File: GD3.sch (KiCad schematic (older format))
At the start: 19 parts, among them IC13 HCPL-316J, IC14 IXDD614PI, P14 CONN_01X03, P15 CONN_01X03

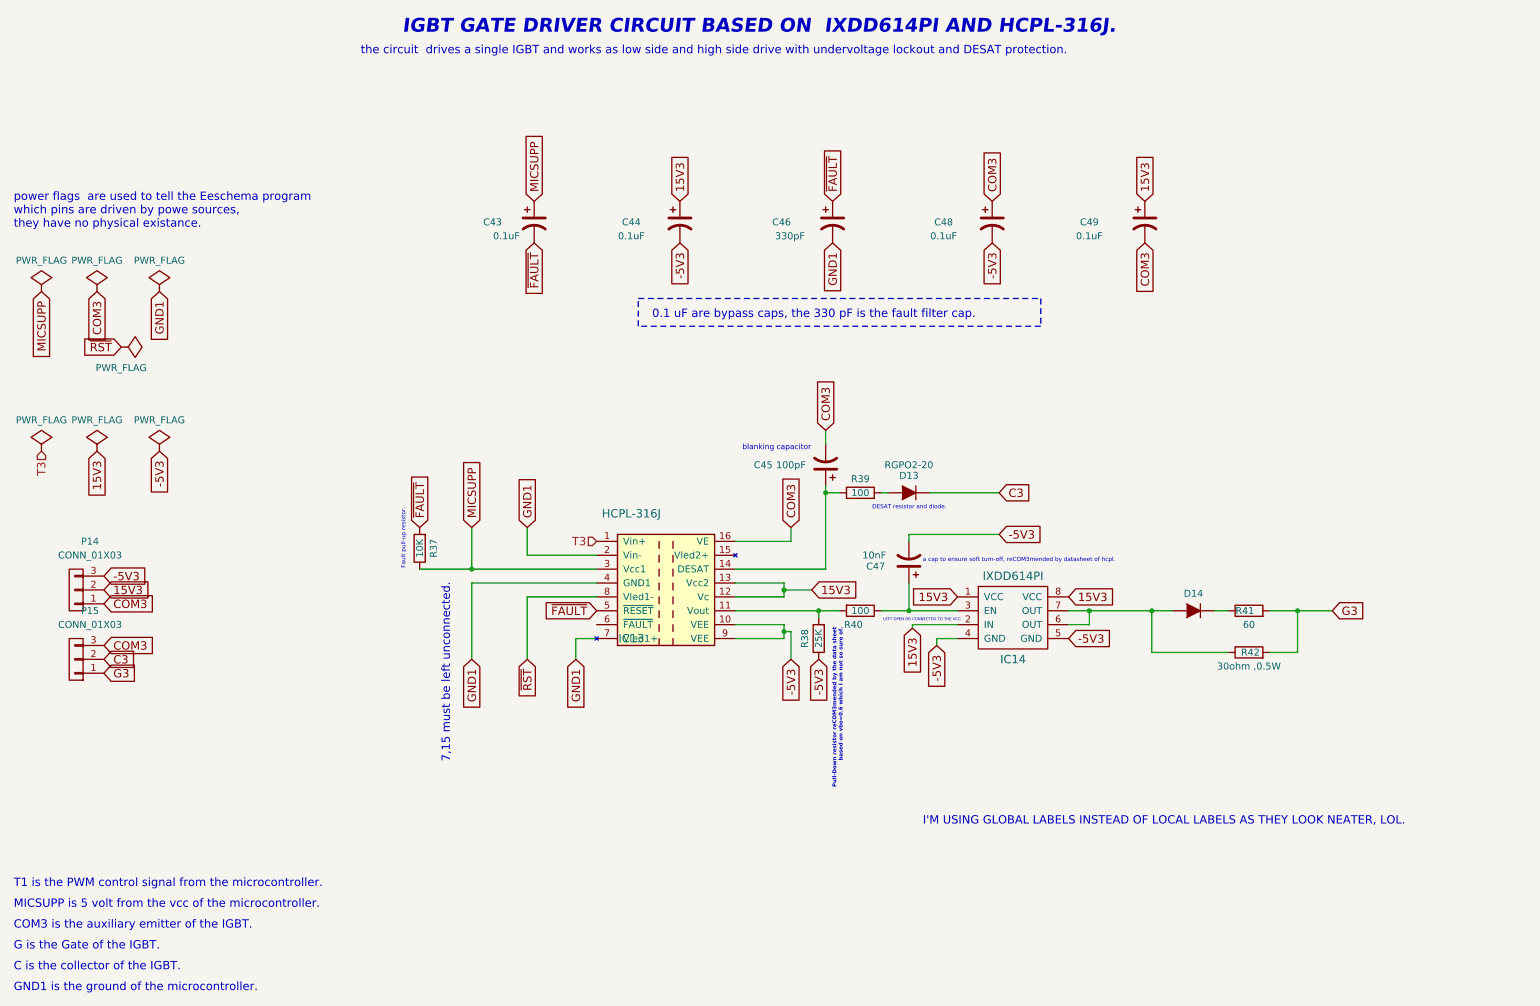
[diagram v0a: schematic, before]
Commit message: packup
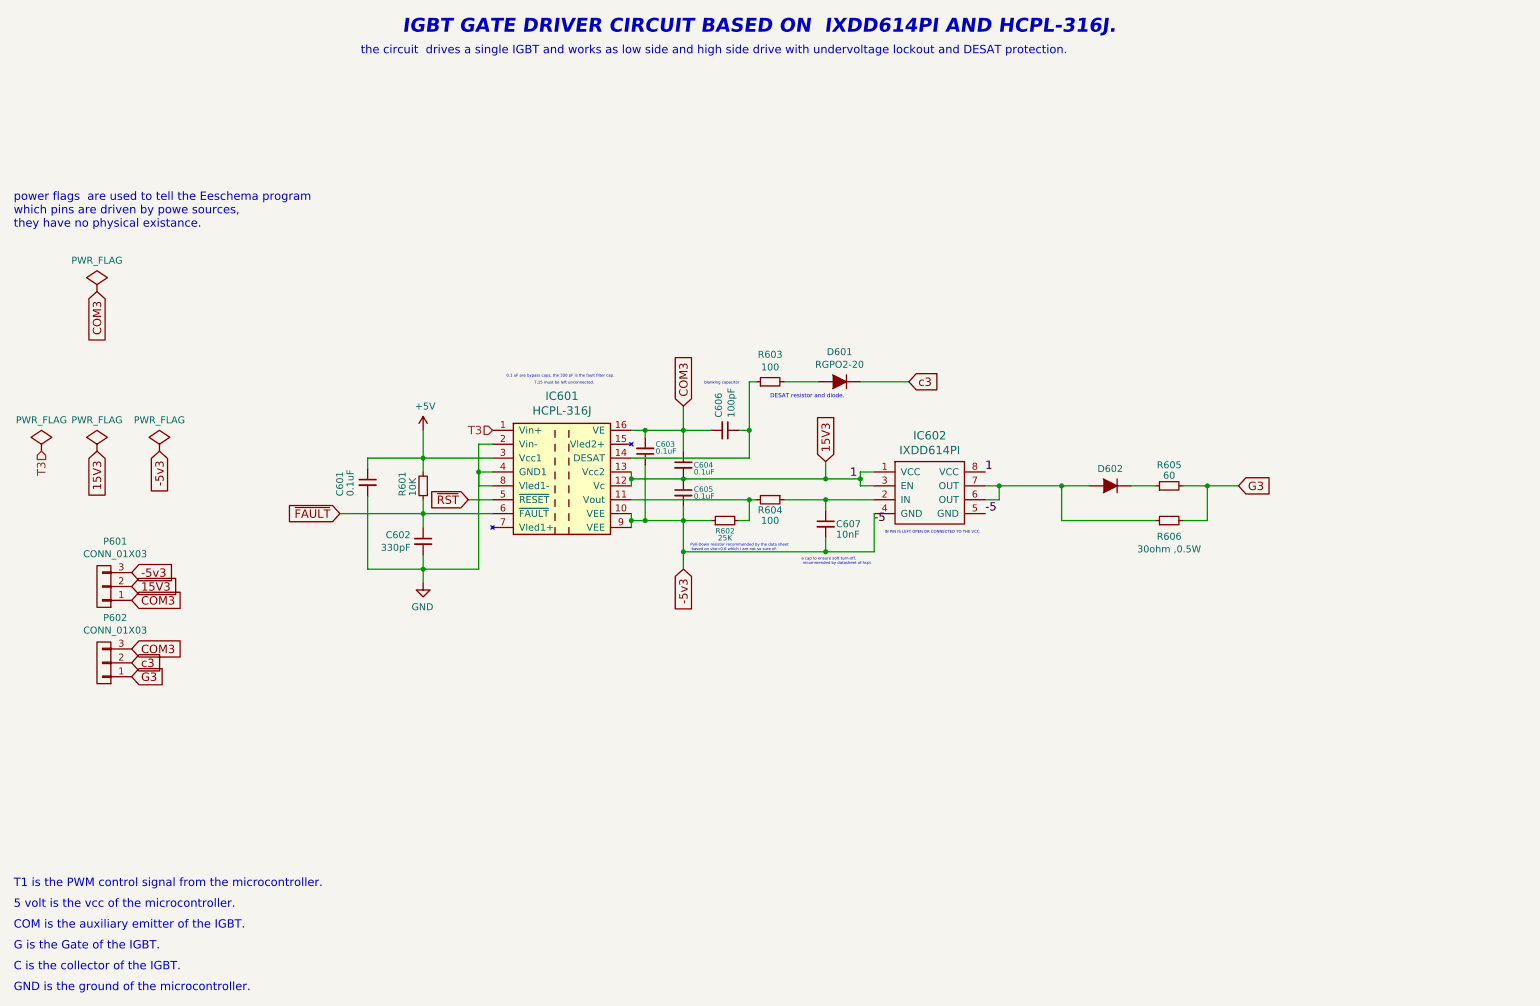
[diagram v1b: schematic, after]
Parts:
- removed C43, C44, C48, C49: 0.1uF, gatedrive:C_Disc, symbol CP1
- removed C45: 100pF, gatedrive:C_Disc, symbol CP1
- removed C46: 330pF, Capacitors_ThroughHole:C_Disc_D3_P2.5, symbol CP1
- removed C47: 10nF, gatedrive:C_Disc, symbol CP1
- removed D13: RGPO2-20, Diodes_ThroughHole:Diode_DO-41_SOD81_Horizontal_RM10, symbol D
- removed D14: ~, Diodes_ThroughHole:Diode_DO-201AD_Horizontal_RM15, symbol D
- removed IC13: HCPL-316J, Housings_SOIC:SOIC-16_7.5x10.3mm_Pitch1.27mm, symbol HCPL-316J
- removed IC14: IXDD614PI, gatedrive:DIP-8_W7.62mm_LongPads, symbol IXDD614PI
- removed P14, P15: CONN_01X03, Pin_Headers:Pin_Header_Angled_1x03, symbol CONN_01X03
- removed R37: 10K, Resistors_ThroughHole:Resistor_Horizontal_RM10mm, symbol R
- removed R38: 25K, Resistors_ThroughHole:Resistor_Horizontal_RM10mm, symbol R
- removed R39, R40: 100, Resistors_ThroughHole:Resistor_Horizontal_RM10mm, symbol R
- removed R41: 60, gatedrive:Resistor_multi, symbol R
- removed R42: 30ohm ,0.5W, gatedrive:Resistor_multi, symbol R
- added C601, C603, C604, C605: 0.1uF, gatedrive:C_Disc, symbol C_Small
- added C602: 330pF, gatedrive:C_Disc, symbol C_Small
- added C606: 100pF, gatedrive:C_Disc, symbol C_Small
- added C607: 10nF, gatedrive:C_Disc, symbol C_Small
- added D601: RGPO2-20, Diodes_ThroughHole:Diode_DO-41_SOD81_Horizontal_RM10, symbol D
- added D602: ~, Diodes_ThroughHole:Diode_DO-201AD_Horizontal_RM15, symbol D
- added IC601: HCPL-316J, Housings_SOIC:SOIC-16_7.5x10.3mm_Pitch1.27mm, symbol HCPL-316J
- added IC602: IXDD614PI, gatedrive:DIP-8_W7.62mm_LongPads, symbol IXDD614PI
- added P601, P602: CONN_01X03, gatedrive:conn, symbol CONN_01X03
- added R601: 10K, Resistors_ThroughHole:Resistor_Horizontal_RM10mm, symbol R_Small
- added R602: 25K, Resistors_ThroughHole:Resistor_Horizontal_RM10mm, symbol R_Small
- added R603, R604: 100, Resistors_ThroughHole:Resistor_Horizontal_RM10mm, symbol R_Small
- added R605: 60, gatedrive:Resistor_multi, symbol R_Small
- added R606: 30ohm ,0.5W, gatedrive:Resistor_multi, symbol R_Small
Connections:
- net 15V3: now also C604.2, C605.1, IC601.12 (Vc), IC601.13 (Vcc2), IC602.1 (VCC), IC602.3 (EN), IC602.8 (VCC), P601.2 (P2)
- net COM3: now also C603.2, C604.1, C606.2, IC601.16 (VE), P601.1 (P1), P602.3 (P3)
- net G3: now also P602.1 (P1), R605.2, R606.2
- net T3: now also IC601.1 (Vin+)
- net ~FAULT: now also C602.1, IC601.6 (~FAULT), R601.1
- net ~RST: now also IC601.5 (~RESET)
- new net: IC601.11 (Vout), R602.2, R604.2
- new net: C606.1, IC601.14 (DESAT), R603.1
- new net: C607.1, IC602.2 (IN), R604.1
- new net: D601.2 (A), R603.2
- new net: D602.1 (K), R605.1
- new net: D602.2 (A), IC602.6 (OUT), IC602.7 (OUT), R606.1
- new net +5V: C601.1, IC601.3 (Vcc1), R601.2
- new net -5v3: C603.1, C605.2, C607.2, IC601.10 (VEE), IC601.9 (VEE), IC602.4 (GND), IC602.5 (GND), P601.3 (P3), R602.1
- new net GND: C601.2, C602.2, IC601.2 (Vin-), IC601.4 (GND1), IC601.8 (Vled1-)
- new net c3: D601.1 (K), P602.2 (P2)
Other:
- note added: "5 volt is the vcc of the microcontroller.\n"
- note added: "COM is the auxiliary emitter of the IGBT."
- note added: "GND is the ground of the microcontroller.\n"
- note added: "IN PIN IS LEFT OPEN OR CONNECTED TO THE VCC."
- note added: "Pull-Down resistor recommended by the data sheet\n based on vbe=0.6 which I am not so sure of."
- note added: "a cap to ensure soft turn-off,\n recommended by datasheet of hcpl."
- note removed: "COM3 is the auxiliary emitter of the IGBT."
- note removed: "Fault pull-up resistor."
- note removed: "GND1 is the ground of the microcontroller.\n"
- note removed: "I'M USING GLOBAL LABELS INSTEAD OF LOCAL LABELS AS THEY LOOK NEATER, LOL."
- note removed: "LEFT OPEN OR CONNECTED TO THE VCC."
- note removed: "MICSUPP is 5 volt from the vcc of the microcontroller.\n"
- note removed: "Pull-Down resistor reCOM3mended by the data sheet\n based on vbe=0.6 which I am not so sure of."
- note removed: "a cap to ensure soft turn-off, reCOM3mended by datasheet of hcpl."

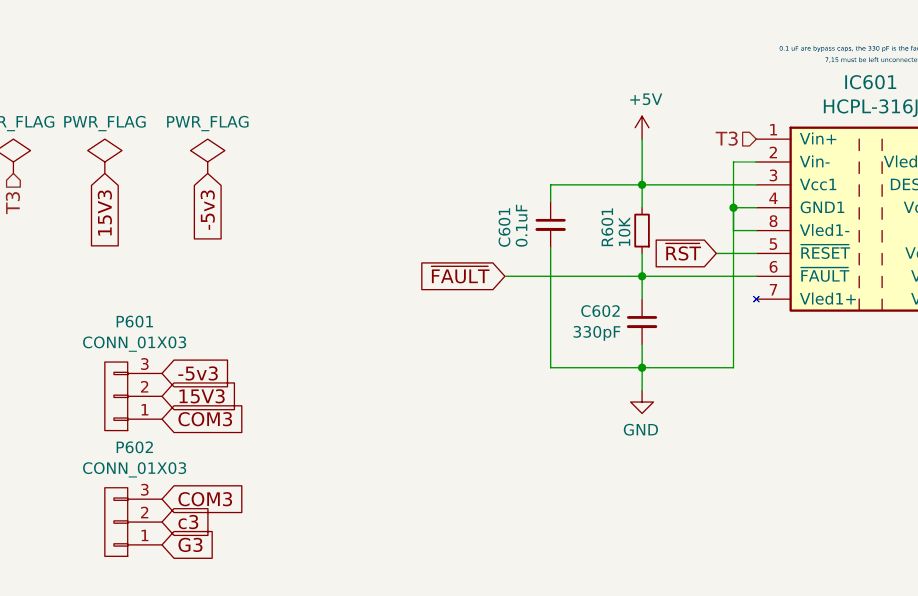
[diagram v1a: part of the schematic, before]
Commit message: parting the protection from the GD
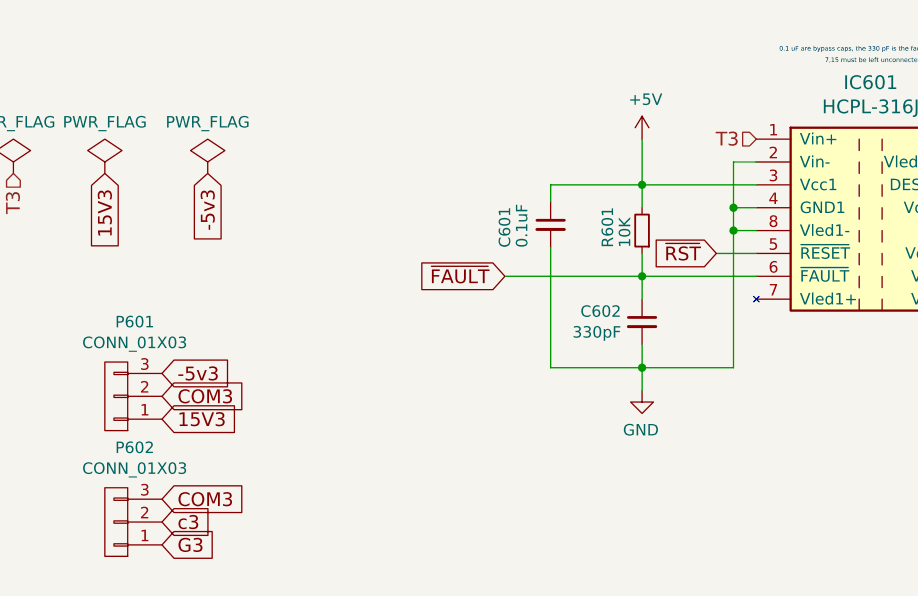
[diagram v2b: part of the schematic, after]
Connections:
- net 15V3: now also P601.1 (P1); no longer P601.2 (P2)
- net COM3: now also P601.2 (P2); no longer P601.1 (P1)
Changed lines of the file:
@@
 IN PIN IS LEFT OPEN OR CONNECTED TO THE VCC.
 $Comp
-L PWR_FLAG #FLG033
+L PWR_FLAG #FLG21
 U 1 1 575FF0FC
 P 1300 3800
-F 0 "#FLG033" H 1300 3895 50  0001 C CNN
+F 0 "#FLG21" H 1300 3895 50  0001 C CNN
 F 1 "PWR_FLAG" H 1300 4024 50  0000 C CNN
 F 2 "" H 1300 3800 50  0000 C CNN
@@
 $EndComp
 $Comp
-L PWR_FLAG #FLG034
+L PWR_FLAG #FLG22
 U 1 1 575FF0FD
 P 1750 3800
-F 0 "#FLG034" H 1750 3895 50  0001 C CNN
+F 0 "#FLG22" H 1750 3895 50  0001 C CNN
 F 1 "PWR_FLAG" H 1750 4024 50  0000 C CNN
 F 2 "" H 1750 3800 50  0000 C CNN
@@
 $EndComp
 $Comp
-L PWR_FLAG #FLG035
+L PWR_FLAG #FLG20
 U 1 1 575FF100
 P 1300 2650
-F 0 "#FLG035" H 1300 2745 50  0001 C CNN
+F 0 "#FLG20" H 1300 2745 50  0001 C CNN
 F 1 "PWR_FLAG" H 1300 2874 50  0000 C CNN
 F 2 "" H 1300 2650 50  0000 C CNN
@@
 $EndComp
 $Comp
-L PWR_FLAG #FLG036
+L PWR_FLAG #FLG19
 U 1 1 575FF101
 P 900 3800
-F 0 "#FLG036" H 900 3895 50  0001 C CNN
+F 0 "#FLG19" H 900 3895 50  0001 C CNN
 F 1 "PWR_FLAG" H 900 4024 50  0000 C CNN
 F 2 "" H 900 3800 50  0000 C CNN
@@
 	5150 4250 5150 4350
 Wire Wire Line
-	5150 3950 5150 4050
-Wire Wire Line
 	6000 3850 5150 3850
 Wire Wire Line
@@
 Wire Wire Line
 	6000 3300 6000 3850
-Connection ~ 7800 4050
 Wire Wire Line
 	7700 4050 8450 4050
@@
 	7700 4150 7800 4150
 Wire Wire Line
-	7800 4150 7800 4050
-Wire Wire Line
 	5150 3650 5725 3650
-Connection ~ 5150 4000
 Wire Wire Line
 	8250 4300 8925 4300
@@
 	-1   0    0    1
 $EndComp
+Text GLabel 1550 4775 2    60   Input ~ 0
+COM3
 Text GLabel 1550 4875 2    60   Input ~ 0
-COM3
-Text GLabel 1550 4775 2    60   Input ~ 0
 15V3
 Text GLabel 1550 5425 2    60   Input ~ 0
@@
 	3975 4150 4150 4150
 $Comp
-L GND #PWR037
+L GND #PWR20
 U 1 1 575FF10A
 P 3650 4750
-F 0 "#PWR037" H 3650 4500 50  0001 C CNN
+F 0 "#PWR20" H 3650 4500 50  0001 C CNN
 F 1 "GND" H 3655 4577 50  0000 C CNN
 F 2 "" H 3650 4750 50  0000 C CNN
@@
 Wire Wire Line
 	4150 3750 4050 3750
-Wire Wire Line
-	4050 3750 4050 4050
-Wire Wire Line
-	4050 4050 4150 4050
-$Comp
-L +5V #PWR038
+$Comp
+L +5V #PWR19
 U 1 1 575FF10B
 P 3650 3650
-F 0 "#PWR038" H 3650 3500 50  0001 C CNN
+F 0 "#PWR19" H 3650 3500 50  0001 C CNN
 F 1 "+5V" H 3665 3823 50  0000 C CNN
 F 2 "" H 3650 3650 50  0000 C CNN
@@
 Connection ~ 3650 4250
 Wire Wire Line
-	4050 3950 4150 3950
-Connection ~ 4050 3950
-Wire Wire Line
 	3650 4550 3650 4750
 Wire Wire Line
-	3250 4650 4050 4650
-Wire Wire Line
-	6550 4225 6550 4150
-Connection ~ 6550 4150
+	4050 4650 3250 4650
 Wire Wire Line
 	3250 3850 3250 3925
@@
 	5525 4200 5525 4650
 Connection ~ 5525 4300
-Connection ~ 5250 3650
-Wire Wire Line
-	5250 3700 5250 3650
 Wire Wire Line
 	5250 3900 5250 4300
 Connection ~ 5250 4300
-Connection ~ 5525 3650
 $Comp
 L C_Small C604
@@
 Connection ~ 6000 3650
 Wire Wire Line
-	5525 3475 5525 3800
-Wire Wire Line
-	4050 4650 4050 3950
+	4050 3750 4050 4650
 Text Label 6725 4000 0    60   ~ 0
 1
@@
 -5
 Wire Wire Line
-	3250 4125 3250 4650
+	3250 4650 3250 4125
 Connection ~ 3650 4650
+Wire Wire Line
+	4150 3950 4050 3950
+Connection ~ 4050 3950
+Wire Wire Line
+	4150 4050 4050 4050
+Connection ~ 4050 4050
+Wire Wire Line
+	5150 3950 5150 4050
+Connection ~ 5150 4000
+Wire Wire Line
+	5250 3700 5250 3650
+Connection ~ 5250 3650
+Wire Wire Line
+	5525 3475 5525 3800
+Connection ~ 5525 3650
+Wire Wire Line
+	6550 4225 6550 4150
+Connection ~ 6550 4150
+Wire Wire Line
+	7800 4150 7800 4050
+Connection ~ 7800 4050
 $EndSCHEMATC
